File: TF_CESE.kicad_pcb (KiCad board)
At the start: 2 copper layers, 85.9 x 137 mm, 25 parts, among them IC1 SN74HC165N, IC2 SN74HC165N, J1 Conn_01x04, J2 Conn_01x03, J3 SD_Card, J4 Conn_01x08, J5 Conn_01x08, J6 Conn_01x02, K1 SANYOU_SRD-05VDC-SL-C, Q1 2N2222A, Q2 S8050, U1 DHT11, U2 RC1602A

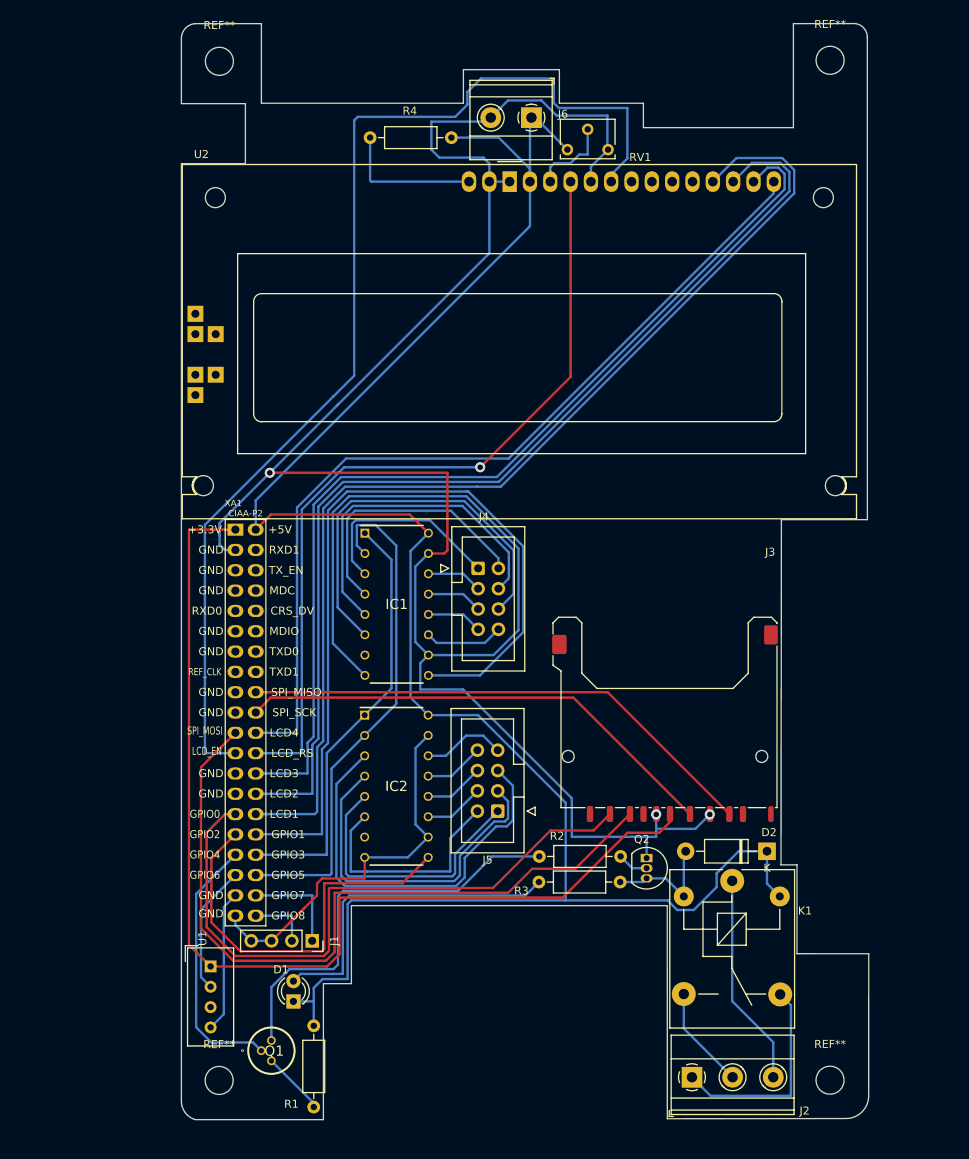
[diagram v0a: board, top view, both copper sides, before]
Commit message: Add files via upload
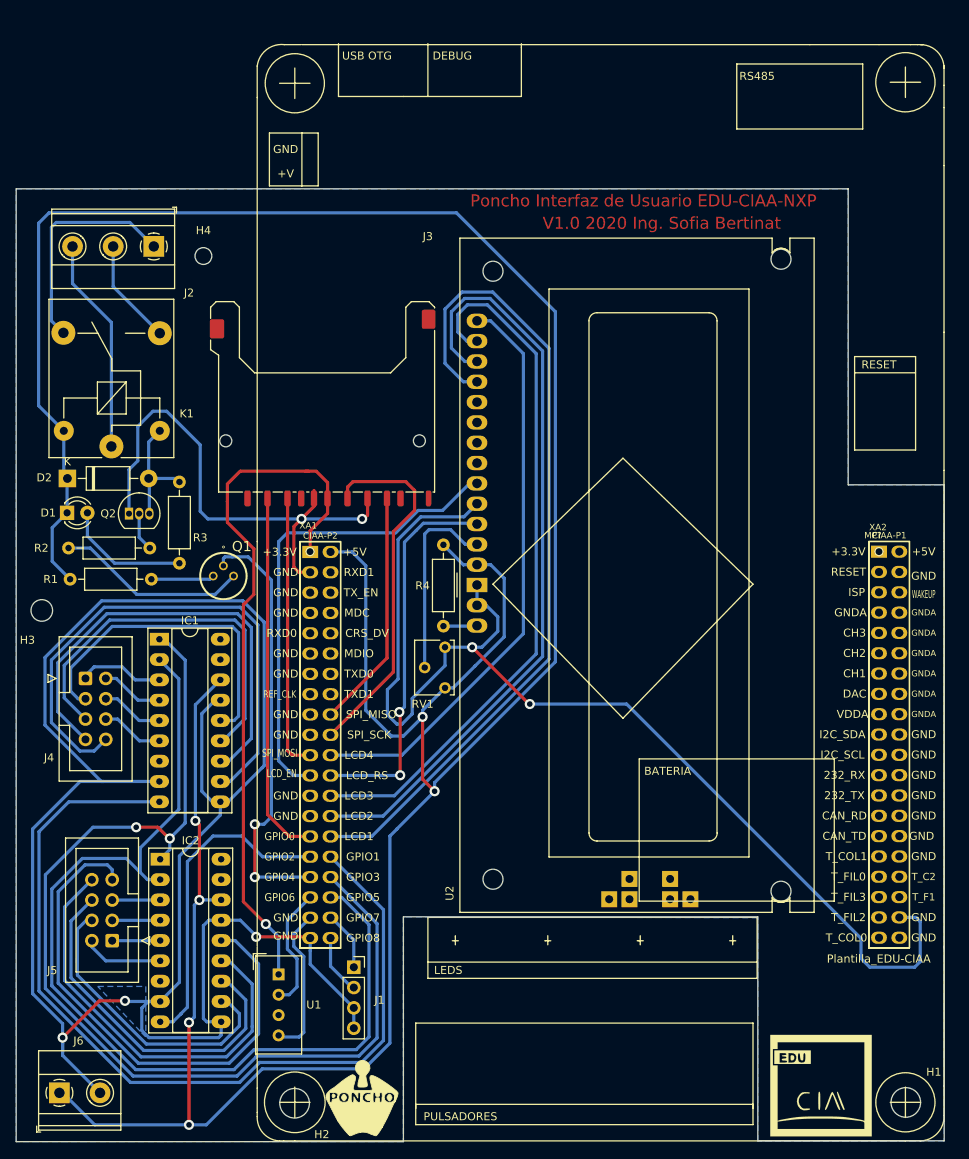
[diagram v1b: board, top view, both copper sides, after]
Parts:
- removed REF** (x4): MountingHole_3.5mm, MountingHole:MountingHole_3.5mm
- added G***: LOGO, Poncho_Esqueleto:Logo_Poncho, F.Cu at (72.3, 169.1)
- added G***: Logo_EDU-CIAA, Poncho_Esqueleto:Logo_EDU-CIAA, F.Cu at (129.7, 167.5)
- added H1: MountingHole, MountingHole:MountingHole_3.7mm, F.Cu at (140.3, 169.6)
- added H2: MountingHole, MountingHole:MountingHole_3.7mm, F.Cu at (63.9, 169.7)
- added H3: MountingHole, MountingHole:MountingHole_2.7mm, F.Cu at (32.3, 108.1)
- added H4: MountingHole, MountingHole:MountingHole_2.1mm, F.Cu at (52.5, 63.8)
- added MP?: Plantilla_EDU-CIAA, Poncho_Esqueleto:Plantilla_EDU-CIAA, F.Cu at (136.9, 100.8)
- added XA2: Conn_Poncho2P_2x_20x2, Poncho_Esqueleto:Conn_Poncho_Derecha, F.Cu at (136.9, 100.8)
- IC1, IC2: footprint KiCad:DIP794W53P254L1930H508Q16N -> Package_DIP:DIP-18_W7.62mm_Socket_LongPads
- moved J6 135.4 mm to (34.5, 168.4), turned to 0 degrees
- moved J2 123.7 mm to (46.3, 62.6), turned to 180 degrees
- moved D2 99.1 mm to (35.5, 91.6), turned to 0 degrees
- moved K1 94.7 mm to (41.0, 87.6), turned to 90 degrees
- moved Q2 77.7 mm to (43.2, 96.0), turned to 0 degrees
- moved R2 70.4 mm to (35.6, 100.3)
- moved RV1 69.0 mm to (82.7, 117.8), turned to 180 degrees
- moved D1 67.3 mm to (35.5, 95.9), turned to 0 degrees
- moved R1 63.6 mm to (35.8, 104.2), turned to 0 degrees
- moved R4 61.7 mm to (82.5, 110.1), turned to 90 degrees
- moved R3 60.1 mm to (49.5, 102.2), turned to 90 degrees
- moved Q1 59.6 mm to (55.0, 103.8), turned to 90 degrees
- moved J3 58.2 mm to (67.4, 81.6)
- moved J4 51.0 mm to (37.8, 116.6)
- moved J5 50.8 mm to (41.1, 149.4)
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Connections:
- net /gpio0 renamed /sd
- net /gpio1 renamed /out1
- net /gpio2 renamed /out2
- net /gpio3 renamed /load
- net /gpio4 renamed /rele
- net /gpio5 renamed /clk
- net Net-(U1-Pad2) renamed /dht11
- net Net-(U1-Pad4) renamed GND1
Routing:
- net +5V: track 251.7 -> 399.6 mm, vias 0 -> 6
- net GND: track 340.8 -> 460.7 mm, vias 3 -> 7
- net /lcdEN: track 141.3 -> 59.9 mm
- net /load: track 53.8 -> 133.8 mm, vias 0 -> 2
- net /clk: track 63.8 -> 123.9 mm
- net /SPI_MOSI: track 93.5 -> 34.6 mm
- net /s00: track 9.88 -> 68.3 mm
- net /s11: track 10.5 -> 66.4 mm
- net Net-(U2-Pad4): track 101.1 -> 48.3 mm, vias 1 -> 2
- net /s01: track 6.98 -> 57.6 mm
- net /s10: track 7.49 -> 54.2 mm
- net /s12: track 51.0 -> 6.06 mm
- net +3.3V: track 131.5 -> 88.7 mm, vias 0 -> 1
- net /s07: track 49.8 -> 7.83 mm
- net /s02: track 6.98 -> 48.6 mm
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- added copper zone on B.Cu, net GND
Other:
- board size 85.9 x 137 mm -> 116 x 119.1 mm
- net class Default: clearance 0.3 -> 0.4; trace_width 0.3 -> 0.4
- rule trace_clearance: 0.3 -> 0.4
- board text added: "Esta placa fue desarrollada en el marco de la materia “Diseño de circuitos impresos” pertenceciente a la Carrera de Especializacion en Sistemas Embebidos de la UBA. Grillas: 1mm, 0.5mm, 0.10mm Vias: 1.27/0.7mm Margen: 0.4 mm Pistas: 0.4mm Distancia a borde: 0.1mm Terminacion: HASL"
- board text added: "Poncho Interfaz de Usuario EDU-CIAA-NXP"
- board text added: "V1.0 2020 Ing. Sofia Bertinat"
